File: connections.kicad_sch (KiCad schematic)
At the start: 31 parts, among them J1 Conn_01x04_Pin, J2 Conn_02x07_Odd_Even, Q1 BSS138, Q2 BSS138, Q3 BSS138

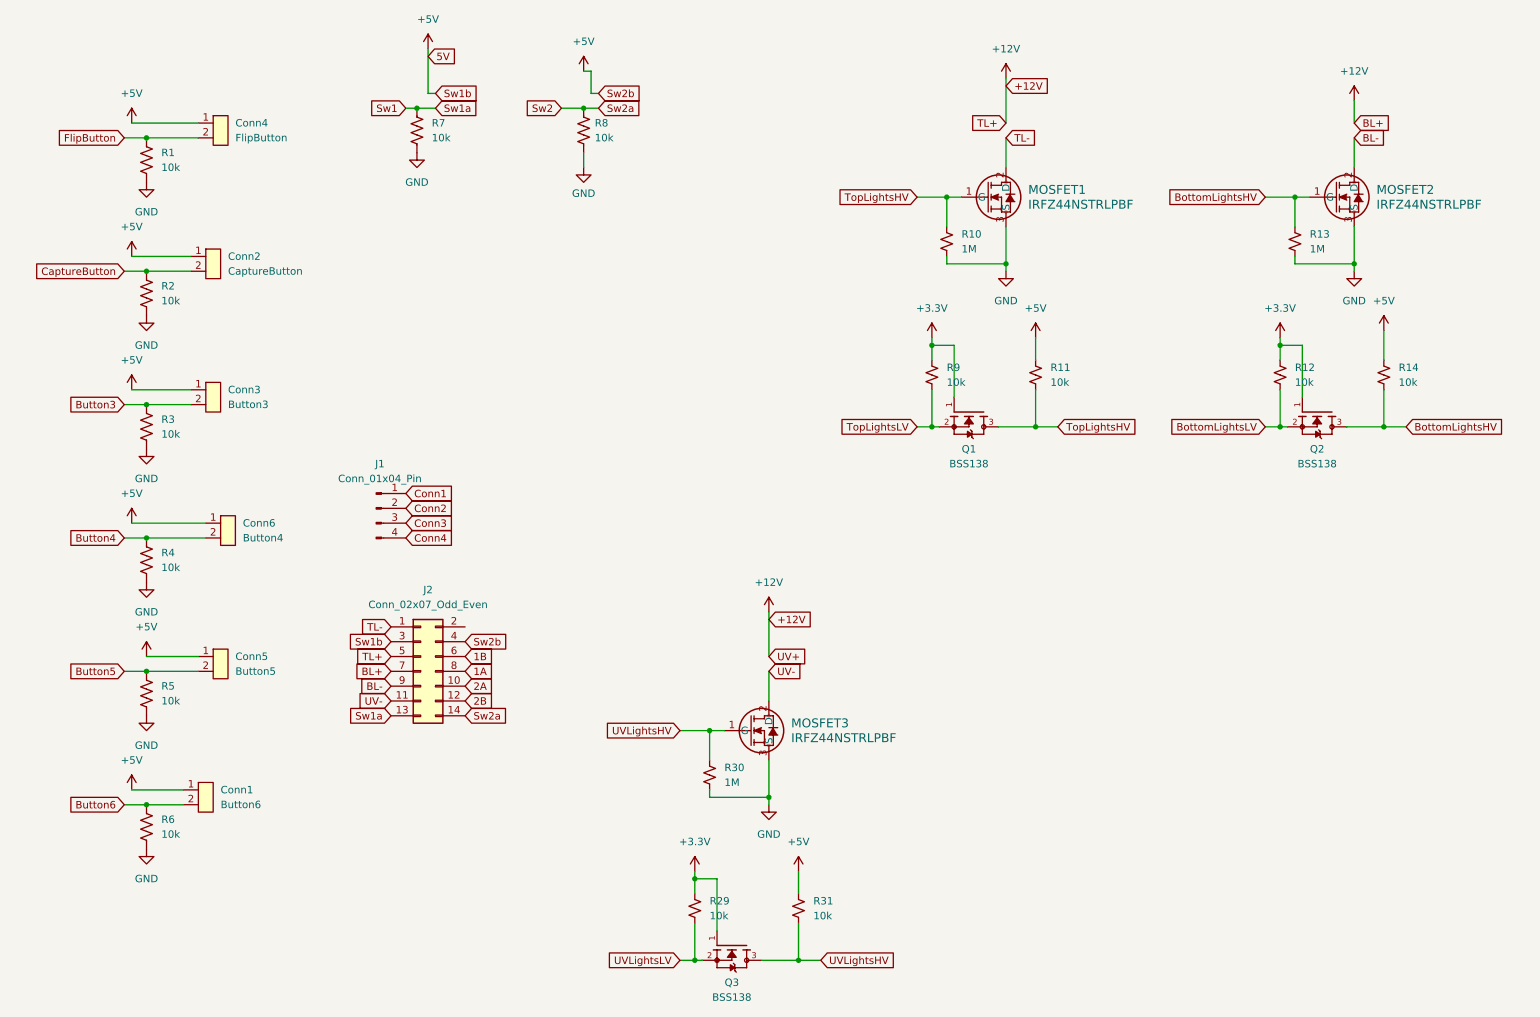
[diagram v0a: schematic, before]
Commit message: Updated board
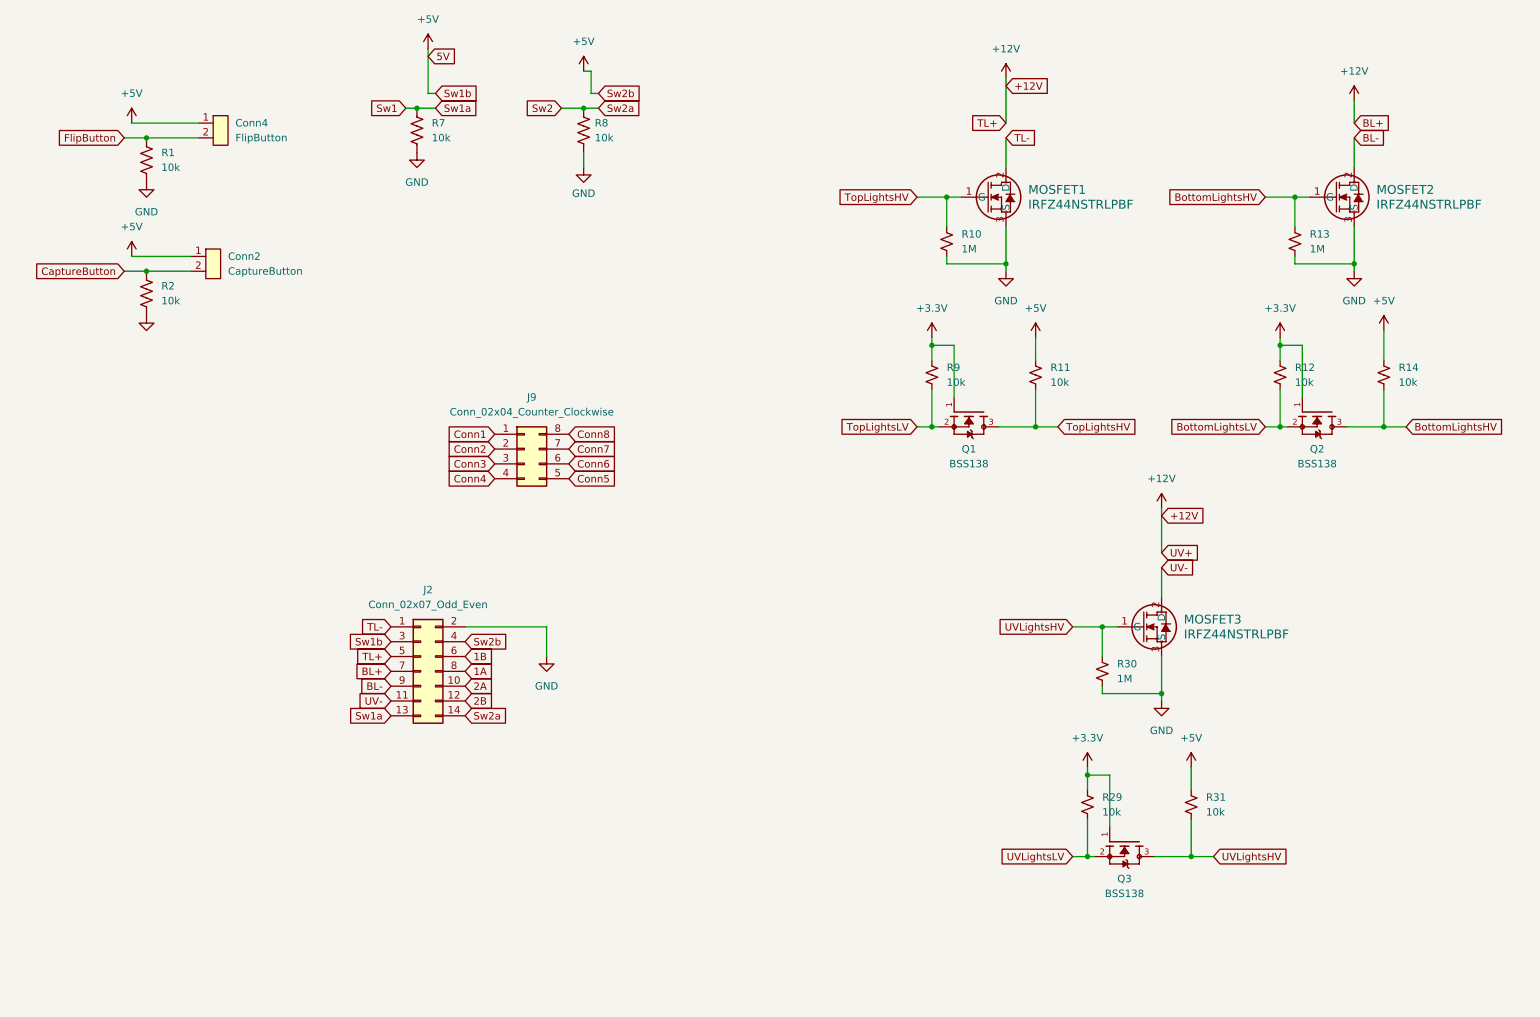
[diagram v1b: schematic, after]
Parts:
- removed Conn1: Button6, Connector_JST:JST_XH_B2B-XH-AM_1x02_P2.50mm_Vertical, symbol Scout_library:B2B_VERT_1.5MM
- removed Conn3: Button3, Connector_JST:JST_XH_B2B-XH-AM_1x02_P2.50mm_Vertical, symbol Scout_library:B2B_VERT_1.5MM
- removed Conn5: Button5, Connector_JST:JST_XH_B2B-XH-AM_1x02_P2.50mm_Vertical, symbol Scout_library:B2B_VERT_1.5MM
- removed Conn6: Button4, Connector_JST:JST_XH_B2B-XH-AM_1x02_P2.50mm_Vertical, symbol Scout_library:B2B_VERT_1.5MM
- removed J1: Conn_01x04_Pin, Connector_PinSocket_2.54mm:PinSocket_1x04_P2.54mm_Vertical, symbol Connector:Conn_01x04_Pin
- removed R3, R4, R5, R6: 10k, Resistor_SMD:R_0603_1608Metric_Pad0.98x0.95mm_HandSolder, symbol Device:R_US
- added J9: Conn_02x04_Counter_Clockwise, Connector_PinSocket_2.54mm:PinSocket_2x04_P2.54mm_Vertical, symbol Connector_Generic:Conn_02x04_Counter_Clockwise
- Conn2, Conn4: LCSC (none) -> C158012; Part Number (none) -> B2B-XH-A-M
- J2: LCSC (none) -> C17661375; Part Number (none) -> 3020-14-0100-00
- MOSFET1, MOSFET2, MOSFET3: LCSC (none) -> C58228; Part Number (none) -> IRFZ44NSTRLPBF
- Q1, Q2, Q3: footprint BSS138:SOT95P240X111-3N -> BSS138W_7_F:SOT-323_DIO; LCSC (none) -> C5250986; Part Number (none) -> BSS138
- R1, R11, R12, R14, R2, R29, R31, R7, R8, R9: LCSC (none) -> C98220; Part Number (none) -> RMCF0603JT10K0
- R10, R13, R30: LCSC (none) -> C4060339; Part Number (none) -> ERJ-3EKF1004V
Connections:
- net Conn1: now also J9.1 (Pin_1)
- net Conn2: now also J9.2 (Pin_2)
- net Conn3: now also J9.3 (Pin_3)
- net Conn4: now also J9.4 (Pin_4)
- net GND: now also J2.2 (Pin_2)
- new net Conn5: J9.5 (Pin_5)
- new net Conn6: J9.6 (Pin_6)
- new net Conn7: J9.7 (Pin_7)
- new net Conn8: J9.8 (Pin_8)
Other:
- moved on the sheet: MOSFET3, Q3, R29, R30, R31
